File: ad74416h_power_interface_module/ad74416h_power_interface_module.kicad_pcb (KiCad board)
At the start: 4 copper layers, 79.3 x 50.2 mm, 132 parts, among them J1 FW-33-03-G-D-085-155, J2 TBP02R1-381-02BE, J3 FW-17-03-G-D-085-155, J4 TBP02R1-381-02BE, T1 ZA9644-AED, U1 MAX17227JATA+, U2 MAX17614ATP+, U3 MAX17570FATA+, U4 ADP1031ACPZ-3-R7, U5 ADUM340E0BRQZ, U6 ADUM340E0BRQZ, U7 ADUM1252AUA+

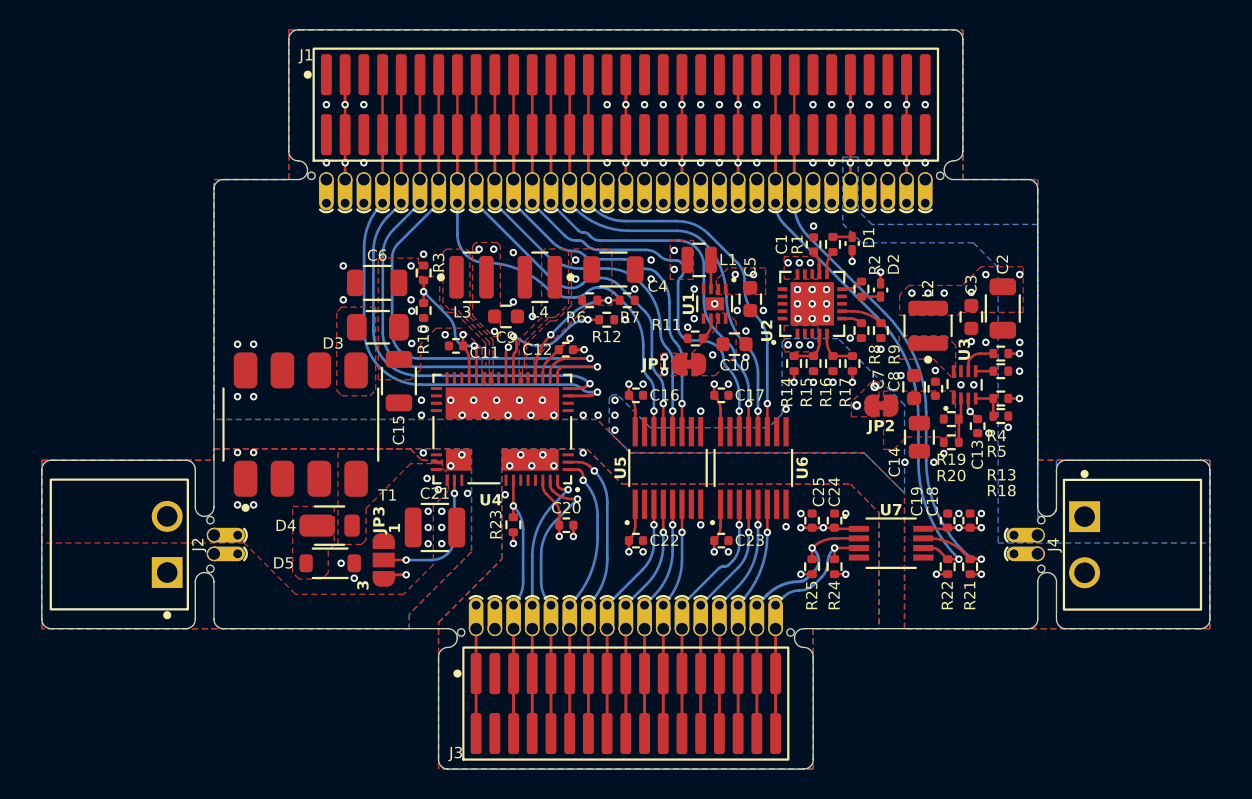
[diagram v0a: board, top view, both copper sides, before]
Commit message: backup
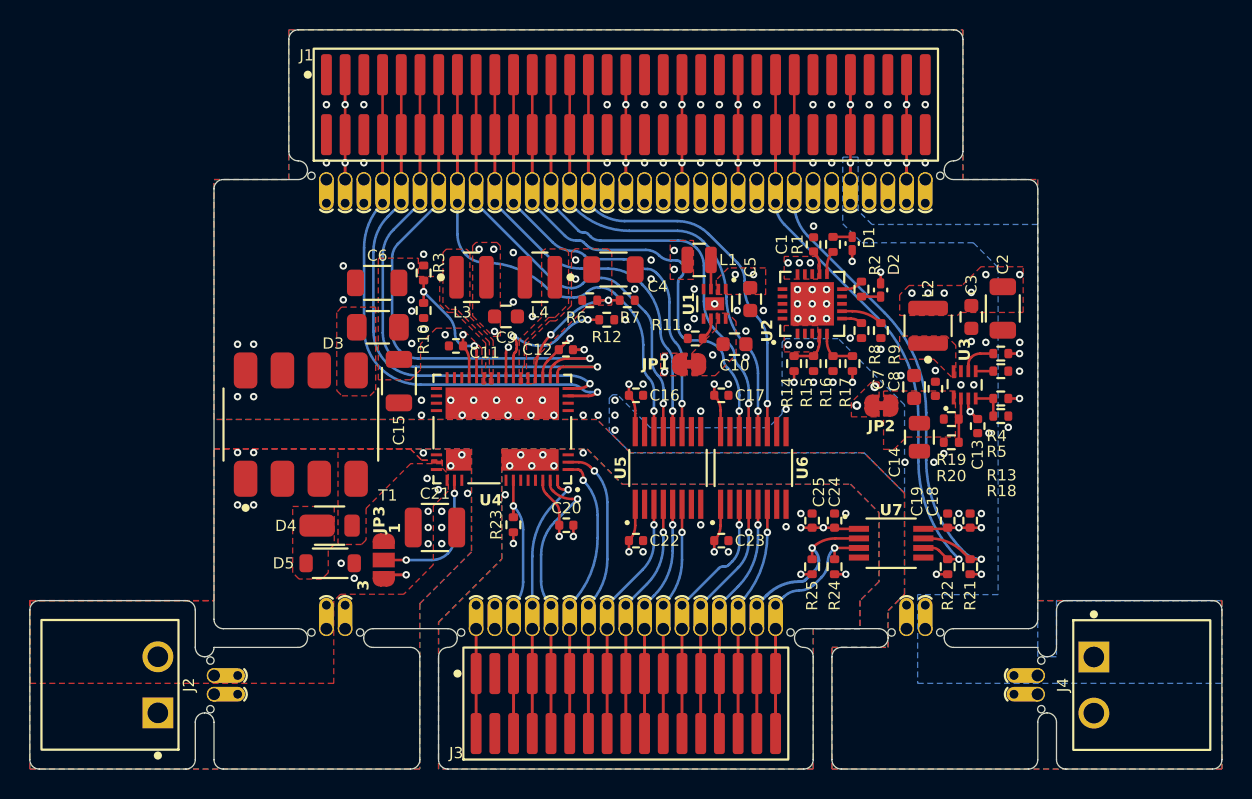
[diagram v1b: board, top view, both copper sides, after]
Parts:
- added MB4: mouse-bite-50mil-200mil, mouse_bite_footprints:mouse-bite-50mil-200mil, F.Cu at (125.1, 120.0)
- added MB6: mouse-bite-50mil-200mil, mouse_bite_footprints:mouse-bite-50mil-200mil, F.Cu at (164.4, 120.0)
- added TP53: TestPoint, test_point_footprints:TestPoint_THTPad_Castelated, F.Cu at (165.1, 119.4)
- added TP54: TestPoint, test_point_footprints:TestPoint_THTPad_Castelated, F.Cu at (163.8, 119.4)
- added TP55: TestPoint, test_point_footprints:TestPoint_THTPad_Castelated, F.Cu at (125.7, 119.4)
- added TP58: TestPoint, test_point_footprints:TestPoint_THTPad_Castelated, F.Cu at (124.4, 119.4)
- moved J2 9.55 mm to (113.0, 123.2)
- moved J4 9.55 mm to (176.5, 123.2)
- moved TP35 9.53 mm to (116.8, 123.8)
- moved TP57 9.53 mm to (172.7, 123.8)
- moved MB1 9.52 mm to (116.2, 123.2)
- moved MB3 9.52 mm to (173.3, 123.2)
- moved TP34 9.52 mm to (116.8, 122.6)
- moved TP56 9.52 mm to (172.7, 122.6)
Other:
- board size 79.3 x 50.2 mm -> 80.9 x 50.2 mm
